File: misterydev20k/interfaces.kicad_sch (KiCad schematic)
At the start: 43 parts, among them J4 Micro_SD_Card_Det1, J5 HDMI_A, SW2 KEY1, SW3 KEY2

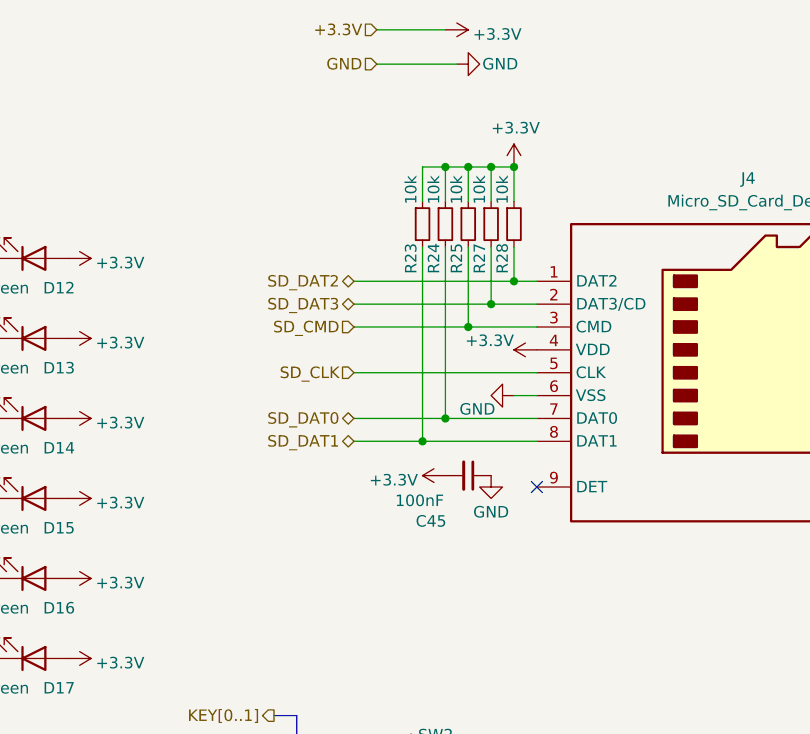
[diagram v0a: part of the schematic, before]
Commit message: Update missing files
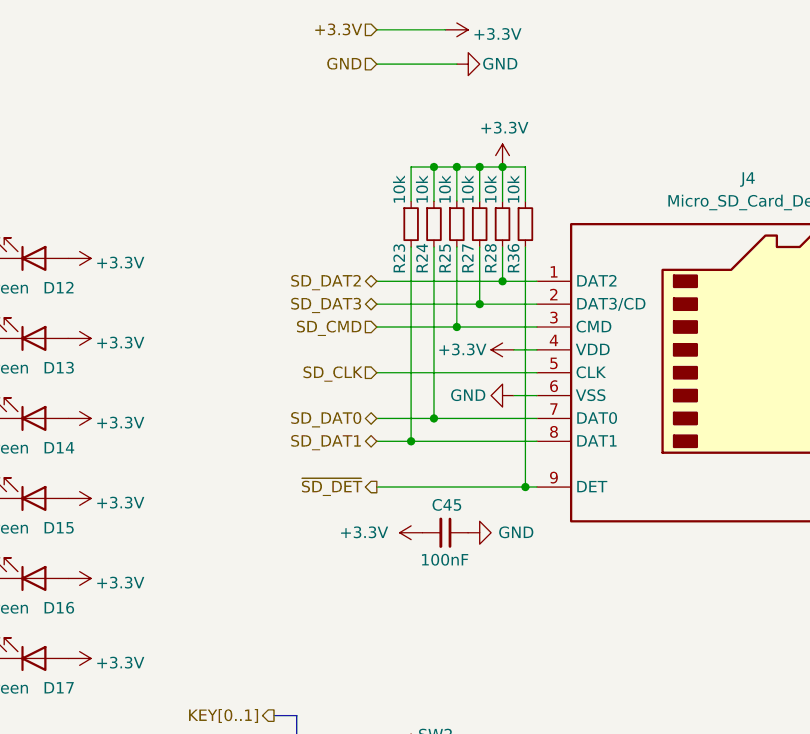
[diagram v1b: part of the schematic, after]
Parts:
- added R36: 10k, Resistor_SMD:R_0402_1005Metric, symbol Device:R_Small
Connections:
- net +3.3V: now also R36.1
- net ~{SD_DET}: now reaches J4.9 (DET)
- net ~{SD_DET}: now also R36.2
- no-connect marks 2 -> 1
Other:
- moved on the sheet: C45, R23, R24, R25, R27, R28
